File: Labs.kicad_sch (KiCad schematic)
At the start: 62 parts, among them J1 PROG_port, J2 USB_C_Receptacle_PowerOnly_6P, Q1 AO3401A, SW1BOOT1 SW_Push, SW2NRST1 SW_Push, U1 STM32F407VGTx, U2 TP4056-42-ESOP8, U3 DW01A, U4 8205A, U5 AMS1117-3.3, Y1 Crystal

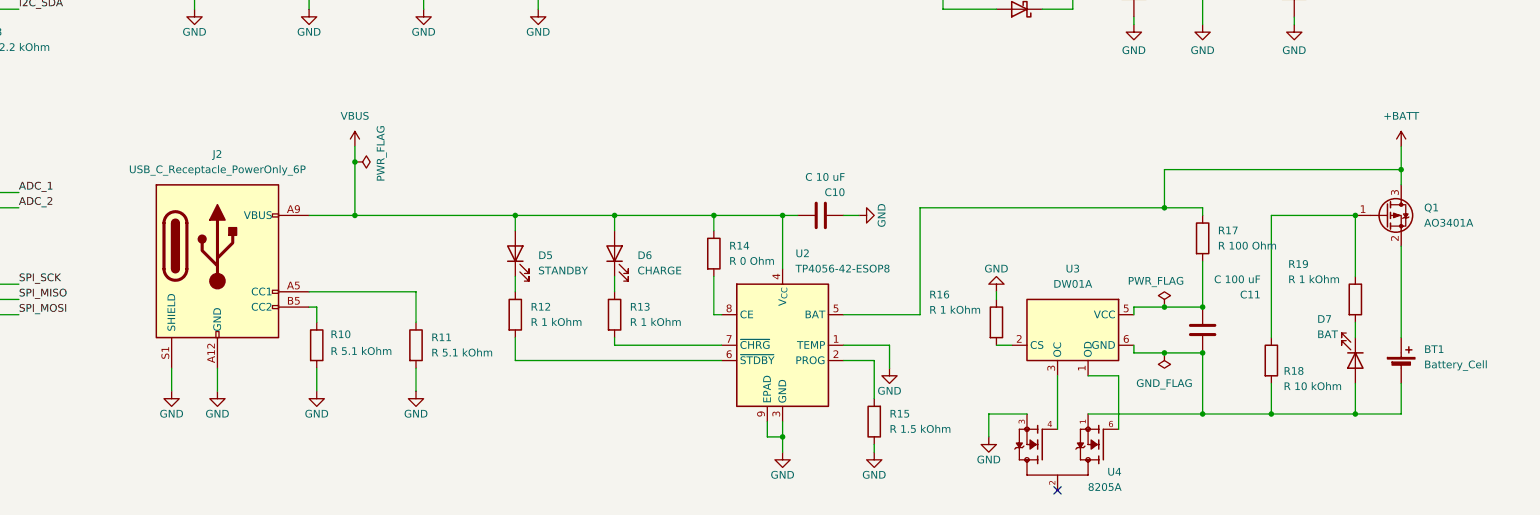
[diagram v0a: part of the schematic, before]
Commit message: feat: add tracing
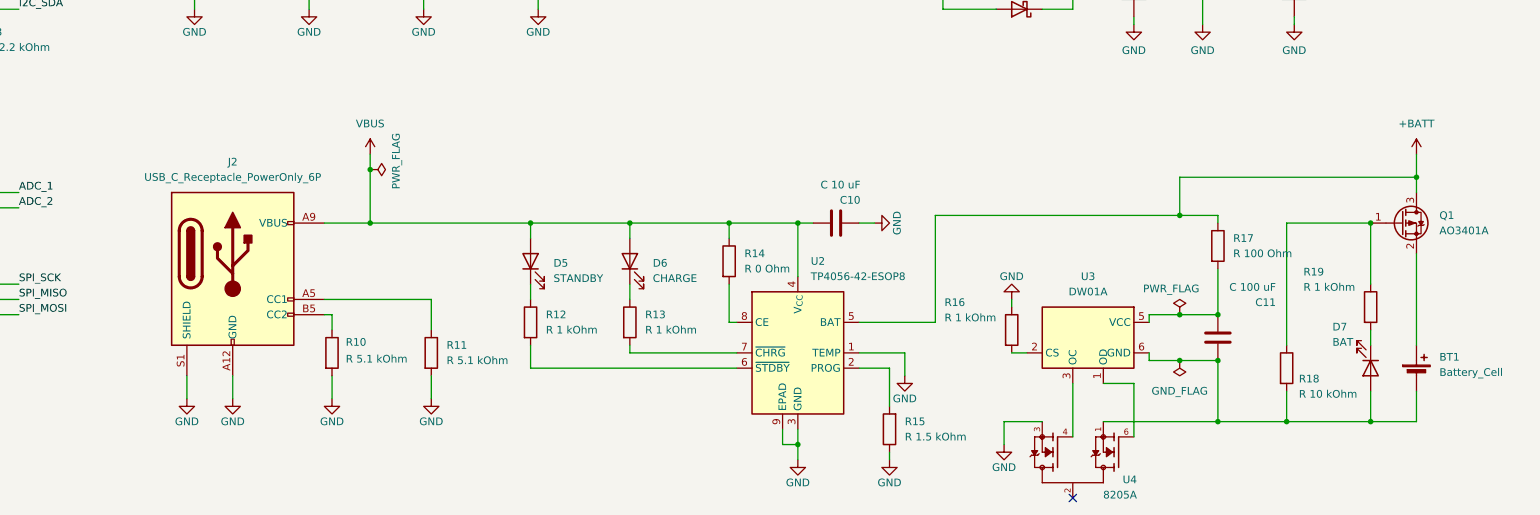
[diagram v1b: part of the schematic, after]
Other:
- moved on the sheet: BT1, C10, C11, D5, D6, D7, J2, Q1, R10, R11, R12, R13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

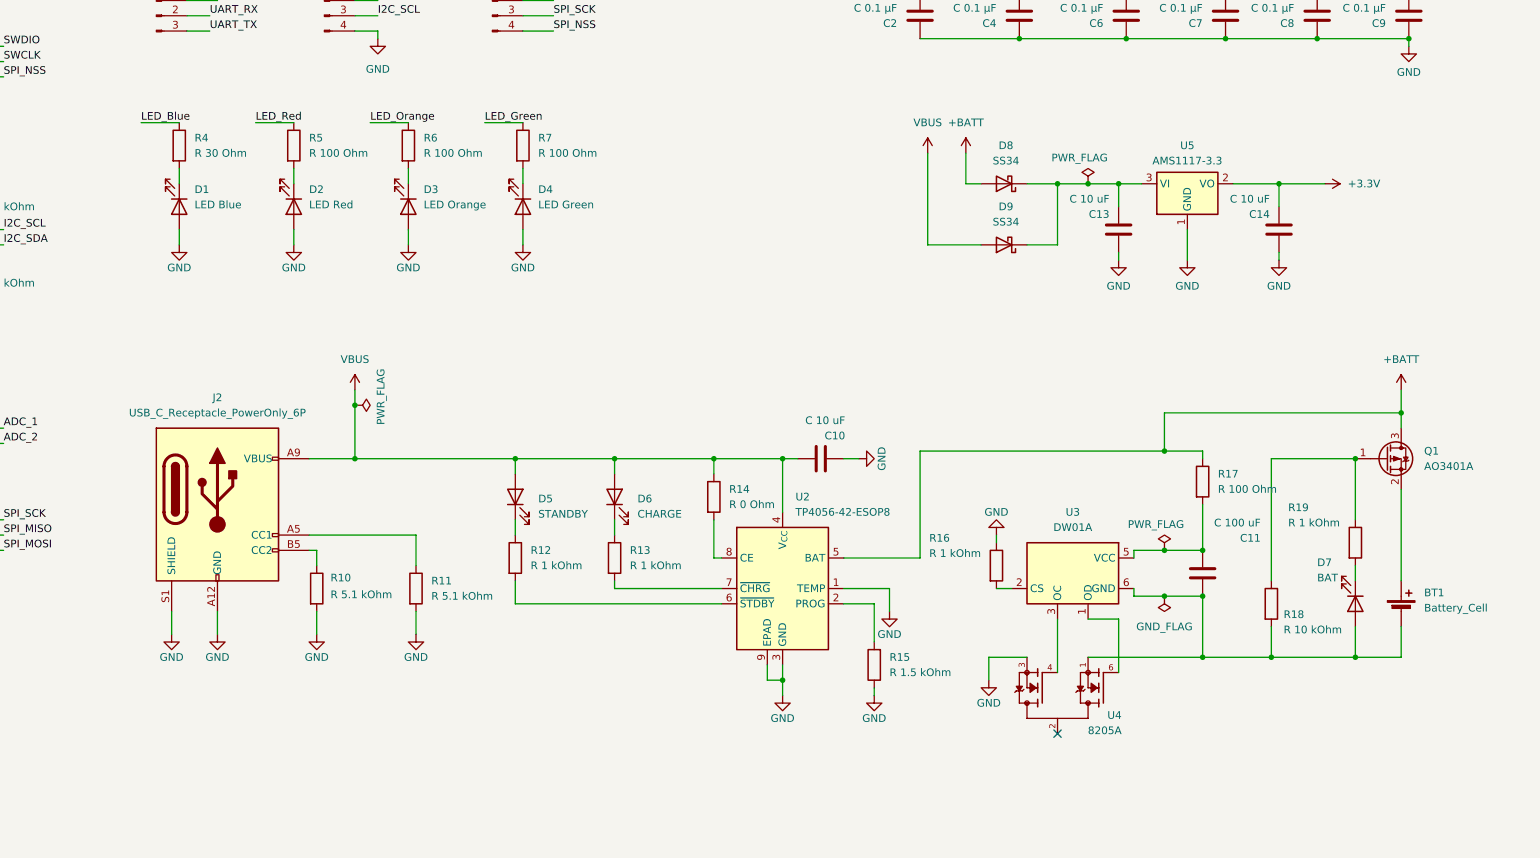
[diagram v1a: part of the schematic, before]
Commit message: fix: minor fixes
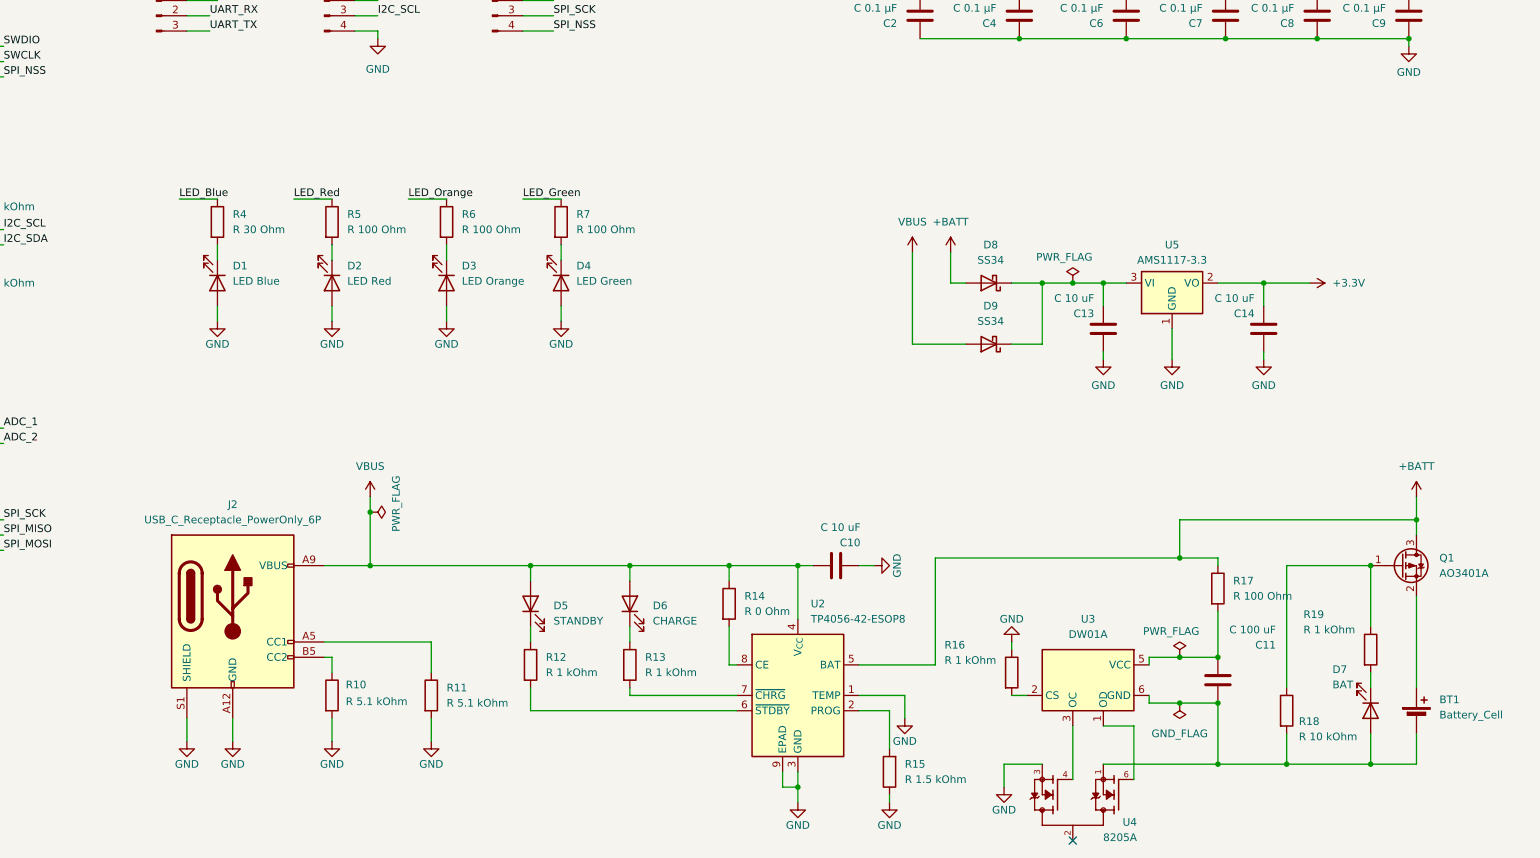
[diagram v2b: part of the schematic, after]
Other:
- moved on the sheet: BT1, C10, C11, C13, C14, D1, D2, D3, D4, D5, D6, D7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
